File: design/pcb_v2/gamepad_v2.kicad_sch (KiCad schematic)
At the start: 26 parts, among them J1 B2B-XH-A, J10 B2B-XH-A, J11 B2B-XH-A, J12 B2B-XH-A, J13 B2B-XH-A, J14 B2B-XH-A, J15 B2B-XH-A, J16 B2B-XH-A, J17 USB_C_Receptacle, J18 Conn_01x02_Female, J2 B2B-XH-A, J3 B2B-XH-A, J4 B2B-XH-A, J5 B2B-XH-A, J6 B2B-XH-A, J7 B2B-XH-A, J8 B2B-XH-A, J9 B2B-XH-A, Q1 MMBT2222A-TP, Q2 MMBT2222A-TP, U1 ESP32-WROOM-32D, U2 CP2104

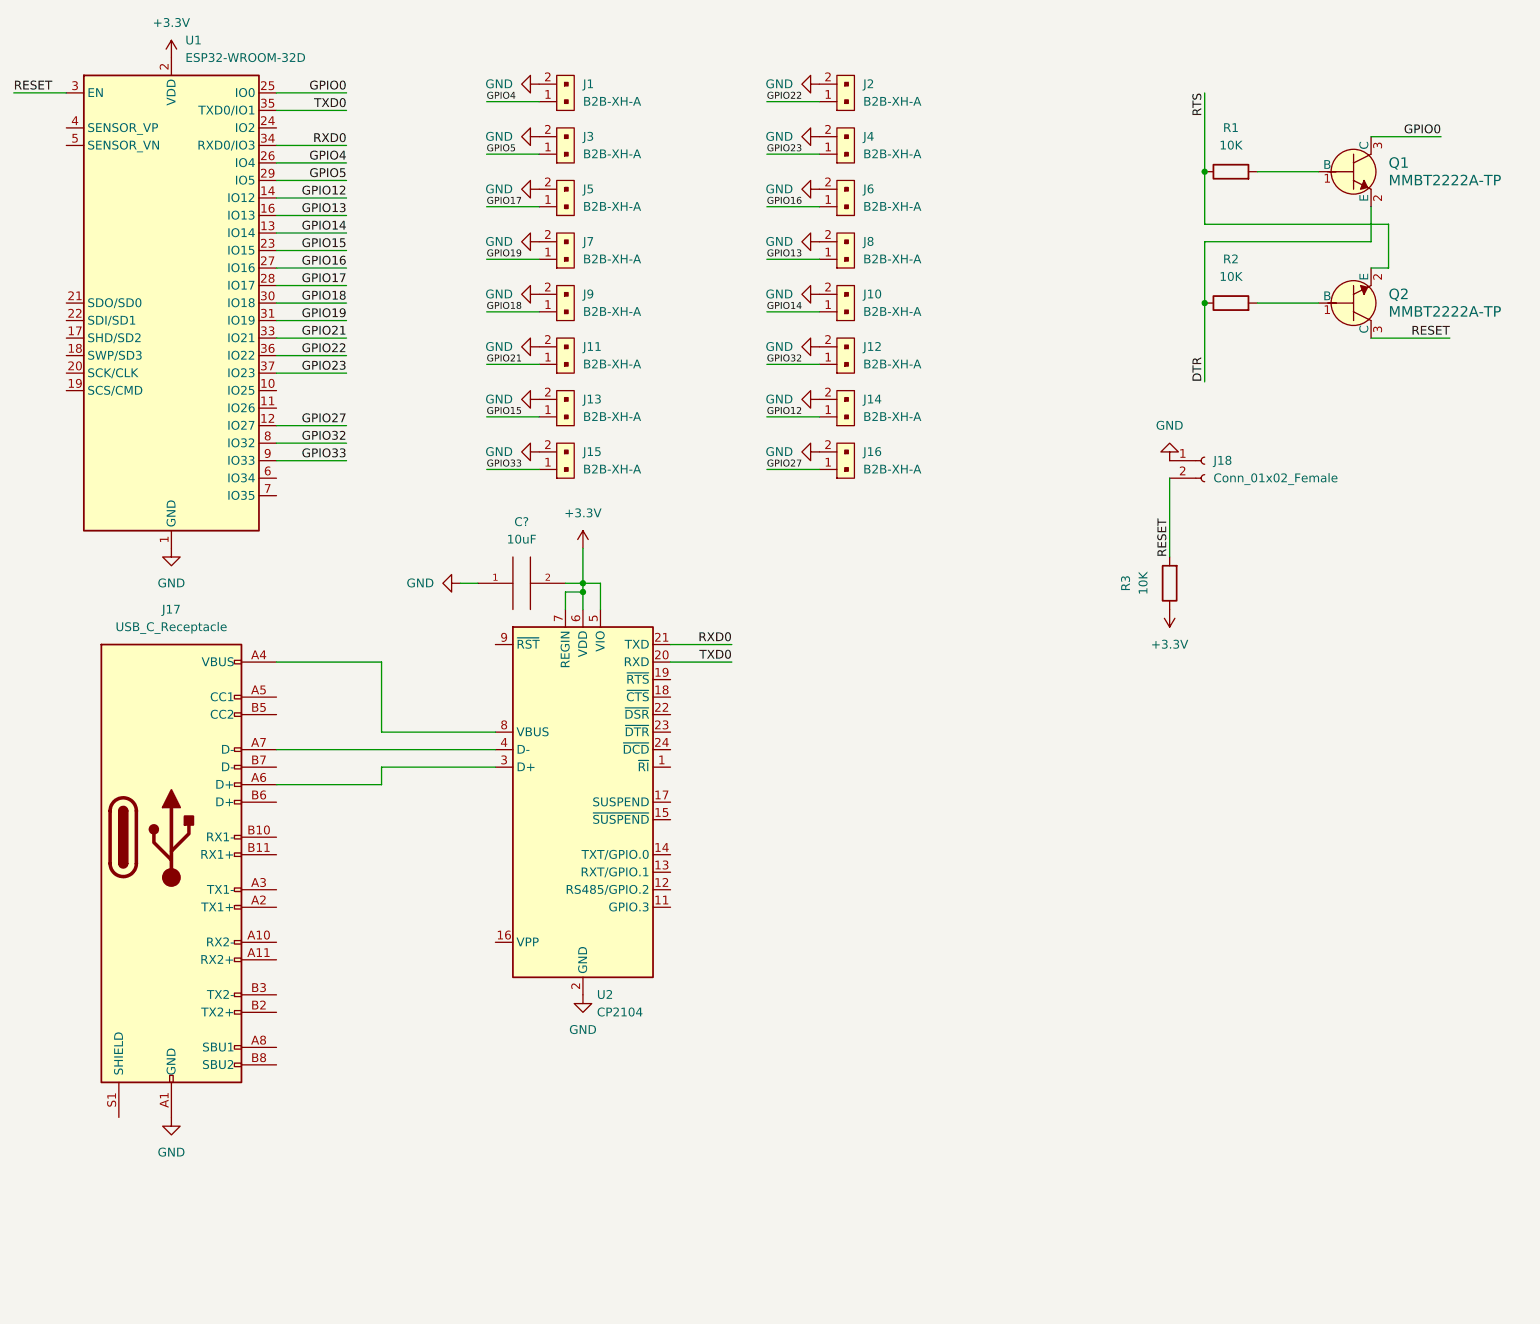
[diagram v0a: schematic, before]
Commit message: I think this is fine
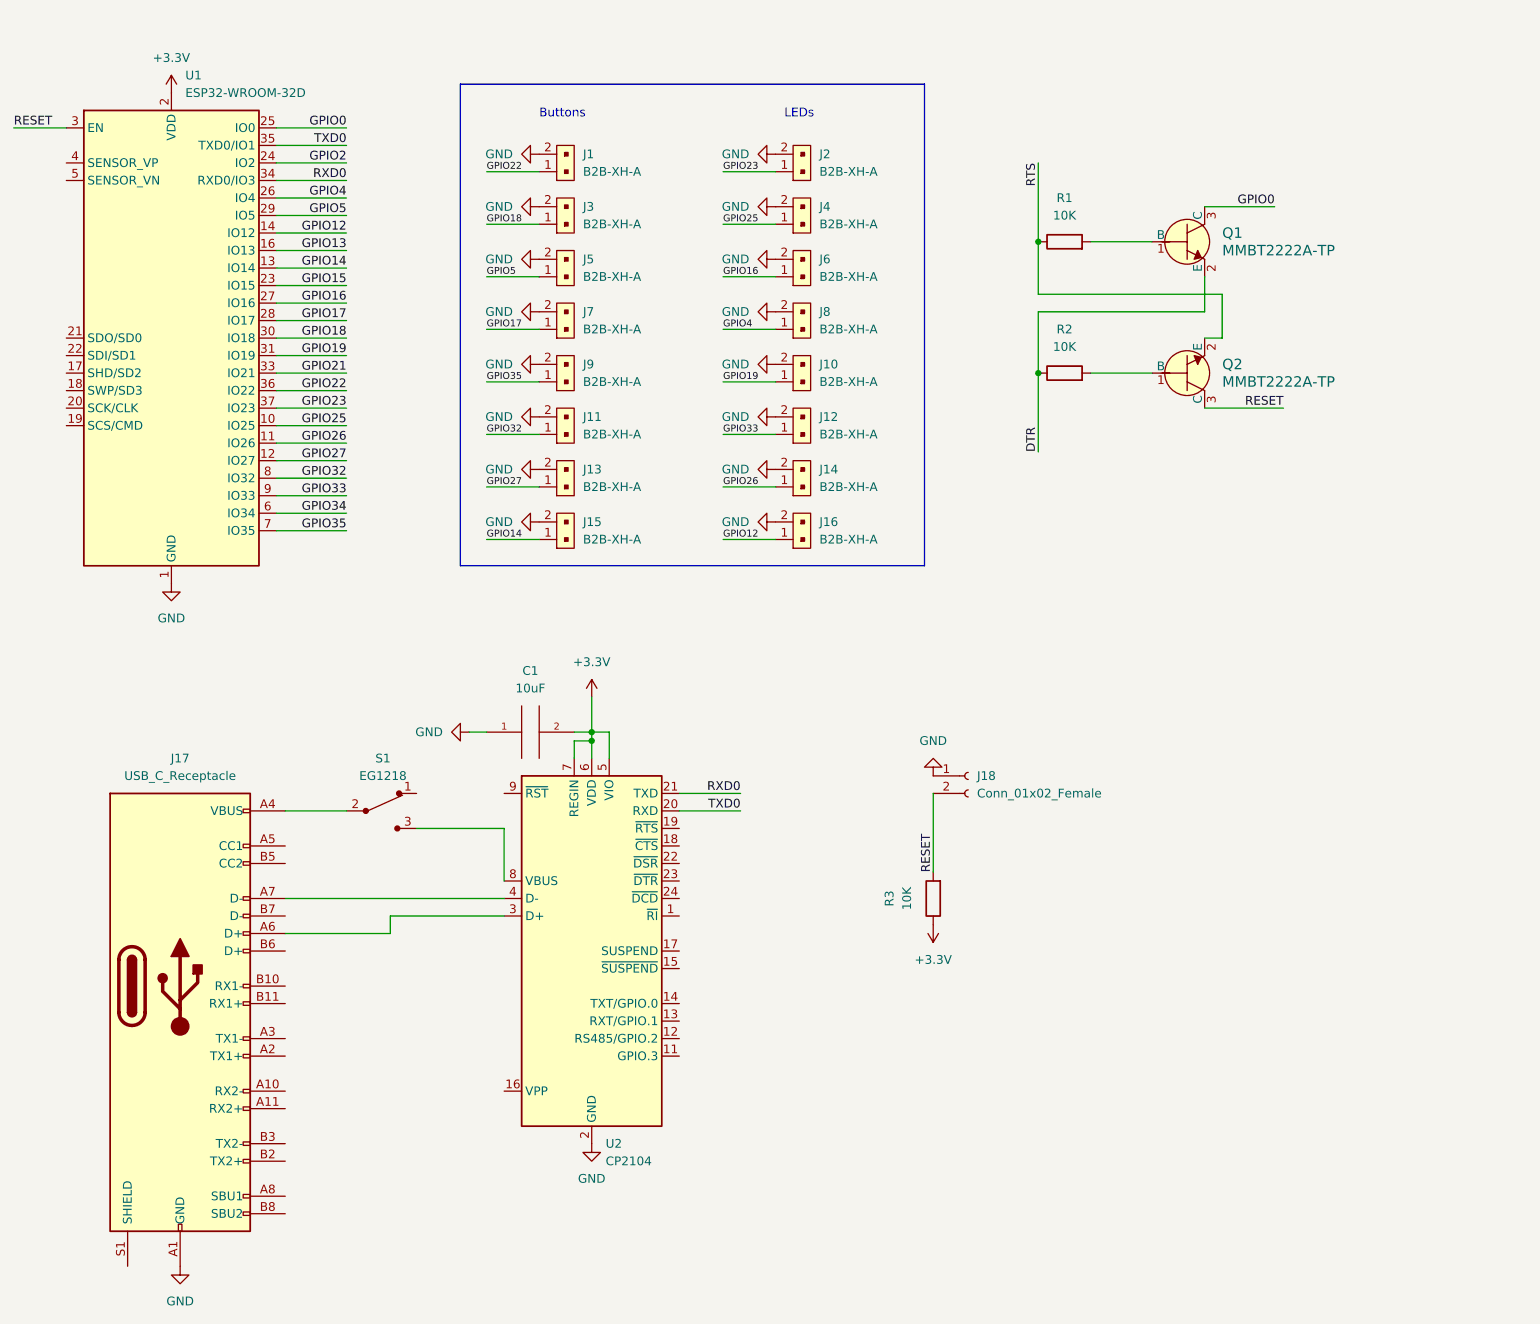
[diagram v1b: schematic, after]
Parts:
- added S1: EG1218, digikey-footprints:Switch_Slide_11.6x4mm_EG1218, symbol dk_Slide-Switches:EG1218
- C1: renamed from C?; footprint (none) -> Capacitor_SMD:C_0603_1608Metric
- J18: footprint Connector_PinHeader_1.00mm:PinHeader_1x02_P1.00mm_Vertical -> Connector_PinHeader_2.54mm:PinHeader_1x02_P2.54mm_Vertical
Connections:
- net GPIO12: now also J16.1; no longer J14.1
- net GPIO13: no longer J8.1
- net GPIO14: now also J15.1; no longer J10.1
- net GPIO15: no longer J13.1
- net GPIO17: now also J7.1; no longer J5.1
- net GPIO18: now also J3.1; no longer J9.1
- net GPIO19: now also J10.1; no longer J7.1
- net GPIO21: no longer J11.1
- net GPIO22: now also J1.1; no longer J2.1
- net GPIO23: now also J2.1; no longer J4.1
- net GPIO27: now also J13.1; no longer J16.1
- net GPIO32: now also J11.1; no longer J12.1
- net GPIO33: now also J12.1; no longer J15.1
- net GPIO4: now also J8.1; no longer J1.1
- net GPIO5: now also J5.1; no longer J3.1
- net at J17.A4 (VBUS), J17.A9 (VBUS), J17.B4 (VBUS)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: now also S1.2; no longer U2.8 (VBUS)
- net GPIO25: now reaches U1.10 (IO25)
- net GPIO25: now also J4.1
- net GPIO26: now reaches U1.11 (IO26)
- net GPIO26: now also J14.1
- net GPIO2: now reaches U1.24 (IO2)
- net GPIO34: now reaches U1.6 (IO34)
- net GPIO35: now reaches U1.7 (IO35)
- net GPIO35: now also J9.1
- new net: S1.3, U2.8 (VBUS)
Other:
- note added: "Buttons"
- note added: "LEDs"
- moved on the sheet: C1, J1, J10, J11, J12, J13, J14, J15, J16, J17, J18, J2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
